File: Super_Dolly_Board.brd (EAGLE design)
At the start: 154.5 x 45 mm, 101 parts, among them J1 10118193-0001LF, J3 SJ1-2503A, J4 RJHSE-5381, J5 SJ1-2503A, J6 SJ1-2503A, P1 TC33X-2, SW1 SKQUDBE010, U1 AT90USB646-MU, U10 IP4234CZ6, U11 AT90USB646-AU, U2 MMDT3904, U3 BTM7755, U4 TS2937CW50, U6 ISL8483, U9 TS2937CW50, X1 3.2X2.5MMCRYSTAL

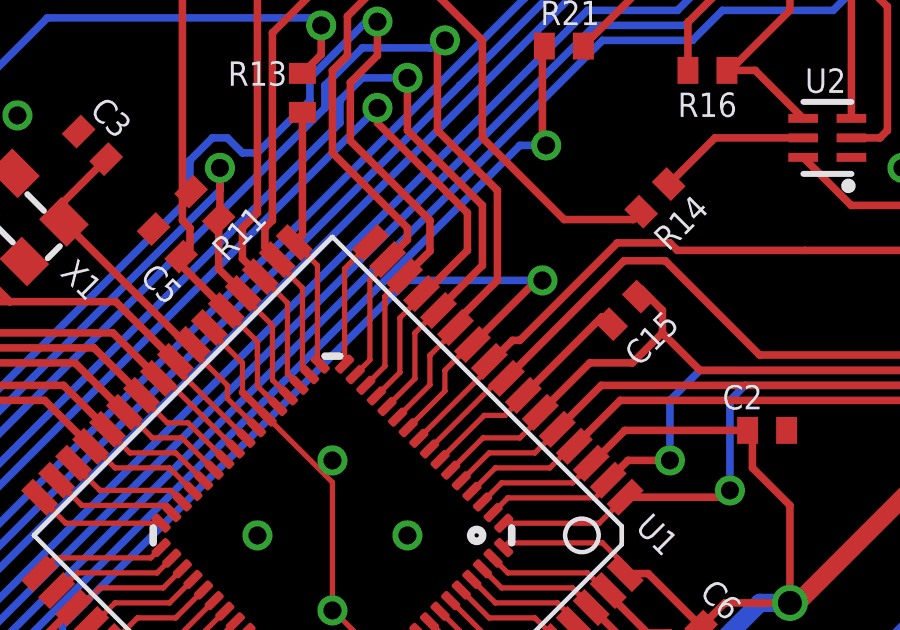
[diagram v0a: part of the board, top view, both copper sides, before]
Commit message: Tagged SDB REV_3
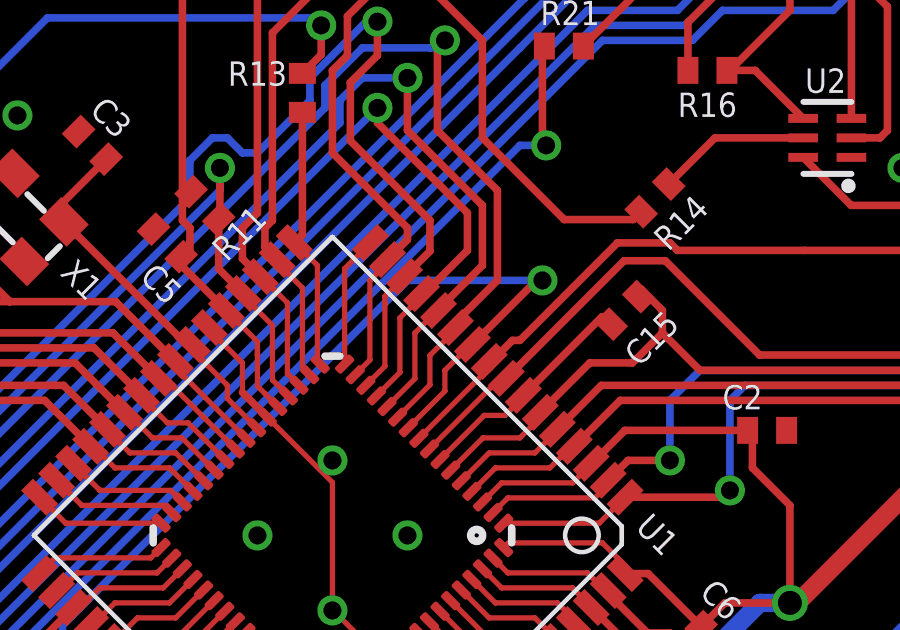
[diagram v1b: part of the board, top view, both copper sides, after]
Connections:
- net N$1 renamed M0_A1
- net N$2 renamed M0_B1
- net N$3 renamed M0_P1
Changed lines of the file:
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@@
 <wire x1="-5.277440625" y1="3.527440625" x2="-2.97255625" y2="3.527440625" width="0.254" layer="1"/>
 <wire x1="-2.97255625" y1="3.527440625" x2="-2.70961875" y2="3.790378125" width="0.254" layer="1"/>
-<wire x1="-11.161521875" y1="2.1923875" x2="-11.161521875" y2="2.088478125" width="0" layer="19" extent="1-1"/>
+<wire x1="-11.161521875" y1="2.088478125" x2="-11.161521875" y2="2.1923875" width="0.254" layer="1"/>
 </signal>
 <signal name="N$5">
@@
 <wire x1="-21.891865625" y1="-6.5934125" x2="-22.758071875" y2="-5.72720625" width="0.1778" layer="1"/>
 </signal>
-<signal name="N$3">
+<signal name="M0_P1">
 <contactref element="R26" pad="1"/>
 <contactref element="U5" pad="27"/>
@@
 <wire x1="49.100003125" y1="-10.65" x2="49.100003125" y2="-8.135" width="0.254" layer="16"/>
 </signal>
-<signal name="N$1">
+<signal name="M0_A1">
 <contactref element="R7" pad="1"/>
 <contactref element="U5" pad="10"/>
@@
 <wire x1="26.85" y1="-19.65" x2="26.85" y2="-17.865" width="0.254" layer="16"/>
 </signal>
-<signal name="N$2">
+<signal name="M0_B1">
 <contactref element="R8" pad="1"/>
 <contactref element="U5" pad="9"/>
@@
 <wire x1="-3.5" y1="2.75" x2="-6.75" y2="-0.5" width="0.254" layer="1"/>
 <wire x1="-6.75" y1="-0.5" x2="-7" y2="-0.5" width="0.254" layer="1"/>
-<wire x1="-7" y1="-0.5" x2="-8" y2="-1.5" width="0.254" layer="1"/>
+<wire x1="-7" y1="-0.5" x2="-7.875" y2="-1.375" width="0.254" layer="1"/>
+<wire x1="-7.875" y1="-1.375" x2="-8" y2="-1.5" width="0.254" layer="1"/>
 <wire x1="2.75" y1="2.5" x2="11" y2="2.5" width="0.254" layer="1"/>
 <via x="14.75" y="2.5" extent="1-16" drill="0.6"/>
@@
 <wire x1="10.75" y1="2.85" x2="11" y2="2.6" width="0.254" layer="1"/>
 <wire x1="11" y1="2.6" x2="11" y2="2.5" width="0.254" layer="1"/>
-<wire x1="-8" y1="-1.5" x2="-7.767409375" y2="-1.41385625" width="0" layer="19" extent="1-1"/>
+<wire x1="-7.767409375" y1="-1.41385625" x2="-7.875" y2="-1.41385625" width="0.254" layer="1"/>
+<wire x1="-7.875" y1="-1.41385625" x2="-7.875" y2="-1.375" width="0.254" layer="1"/>
 </signal>
 <signal name="PE2">
